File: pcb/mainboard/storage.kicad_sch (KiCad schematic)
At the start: 6 parts, among them J401 MICRO_SD(TFC-WPAPR-08), J402 Bus_M.2_Socket_B

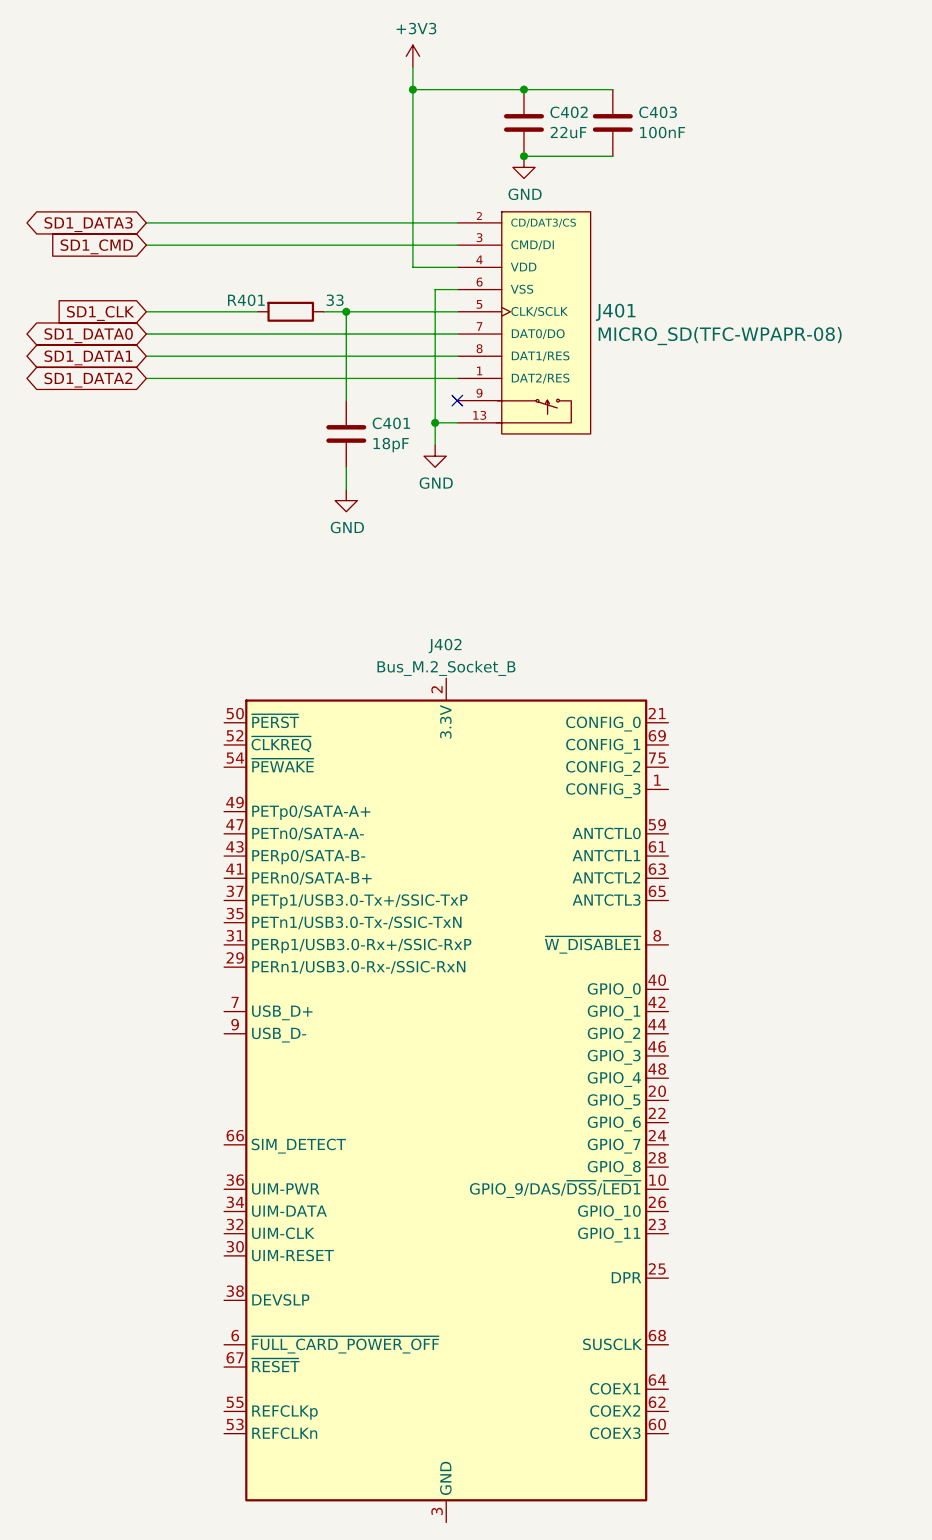
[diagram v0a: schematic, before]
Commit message: - pcb: finishing layout r0p1
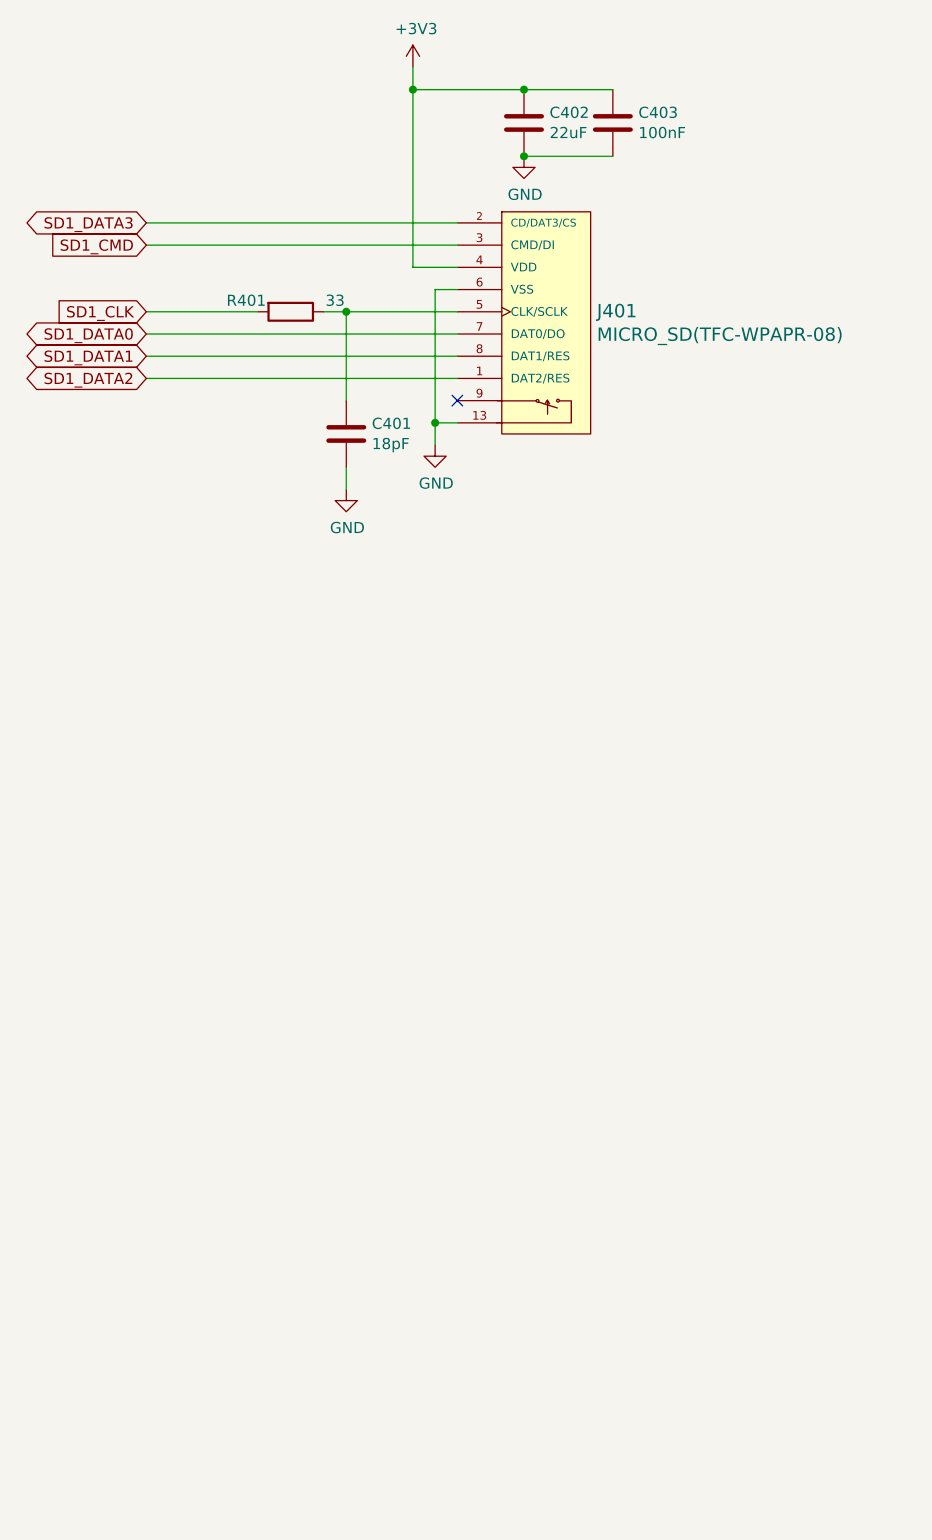
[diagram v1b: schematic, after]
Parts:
- removed J402: Bus_M.2_Socket_B, footprints:M2_BKEY, symbol Connector:Bus_M.2_Socket_B
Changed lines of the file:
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@@
-    (pin "9")
-  )
-  (symbol (lib_id "Connector:Bus_M.2_Socket_B") (at 161.29 191.77 0) (unit 1)
-    (in_bom yes) (on_board yes) (fields_autoplaced)
-    (property "Reference" "J402" (id 0) (at 161.29 139.7 0))
-    (property "Value" "Bus_M.2_Socket_B" (id 1) (at 161.29 142.24 0))
-    (property "Footprint" "footprints:M2_BKEY" (id 2) (at 161.29 165.1 0)
-      (effects (font (size 1.27 1.27)) hide)
-    )
-    (property "Datasheet" "http://read.pudn.com/downloads794/doc/project/3133918/PCIe_M.2_Electromechanical_Spec_Rev1.0_Final_11012013_RS_Clean.pdf#page=154" (id 3) (at 161.29 165.1 0)
-      (effects (font (size 1.27 1.27)) hide)
-    )
-    (pin "1")
-    (pin "10")
-    (pin "11")
-    (pin "2")
-    (pin "20")
-    (pin "21")
-    (pin "22")
-    (pin "23")
-    (pin "24")
-    (pin "25")
-    (pin "26")
-    (pin "27")
-    (pin "28")
-    (pin "29")
-    (pin "3")
-    (pin "30")
-    (pin "31")
-    (pin "32")
-    (pin "33")
-    (pin "34")
-    (pin "35")
-    (pin "36")
-    (pin "37")
-    (pin "38")
-    (pin "39")
-    (pin "4")
-    (pin "40")
-    (pin "41")
-    (pin "42")
-    (pin "43")
-    (pin "44")
-    (pin "45")
-    (pin "46")
-    (pin "47")
-    (pin "48")
-    (pin "49")
-    (pin "5")
-    (pin "50")
-    (pin "51")
-    (pin "52")
-    (pin "53")
-    (pin "54")
-    (pin "55")
-    (pin "56")
-    (pin "57")
-    (pin "58")
-    (pin "59")
-    (pin "6")
-    (pin "60")
-    (pin "61")
-    (pin "62")
-    (pin "63")
-    (pin "64")
-    (pin "65")
-    (pin "66")
-    (pin "67")
-    (pin "68")
-    (pin "69")
-    (pin "7")
-    (pin "70")
-    (pin "71")
-    (pin "72")
-    (pin "73")
-    (pin "74")
-    (pin "75")
-    (pin "8")
     (pin "9")
   )
